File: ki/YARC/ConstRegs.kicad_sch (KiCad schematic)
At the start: 11 parts, among them U91 74HC245, U92 74LS157, U93 74LS32, U94 74HC245, U95 74HC245, U96 74LS32, U96A1 74LS32, U96B1 74LS32, U97 74HC00, U98 74HC245, U99 74HC245

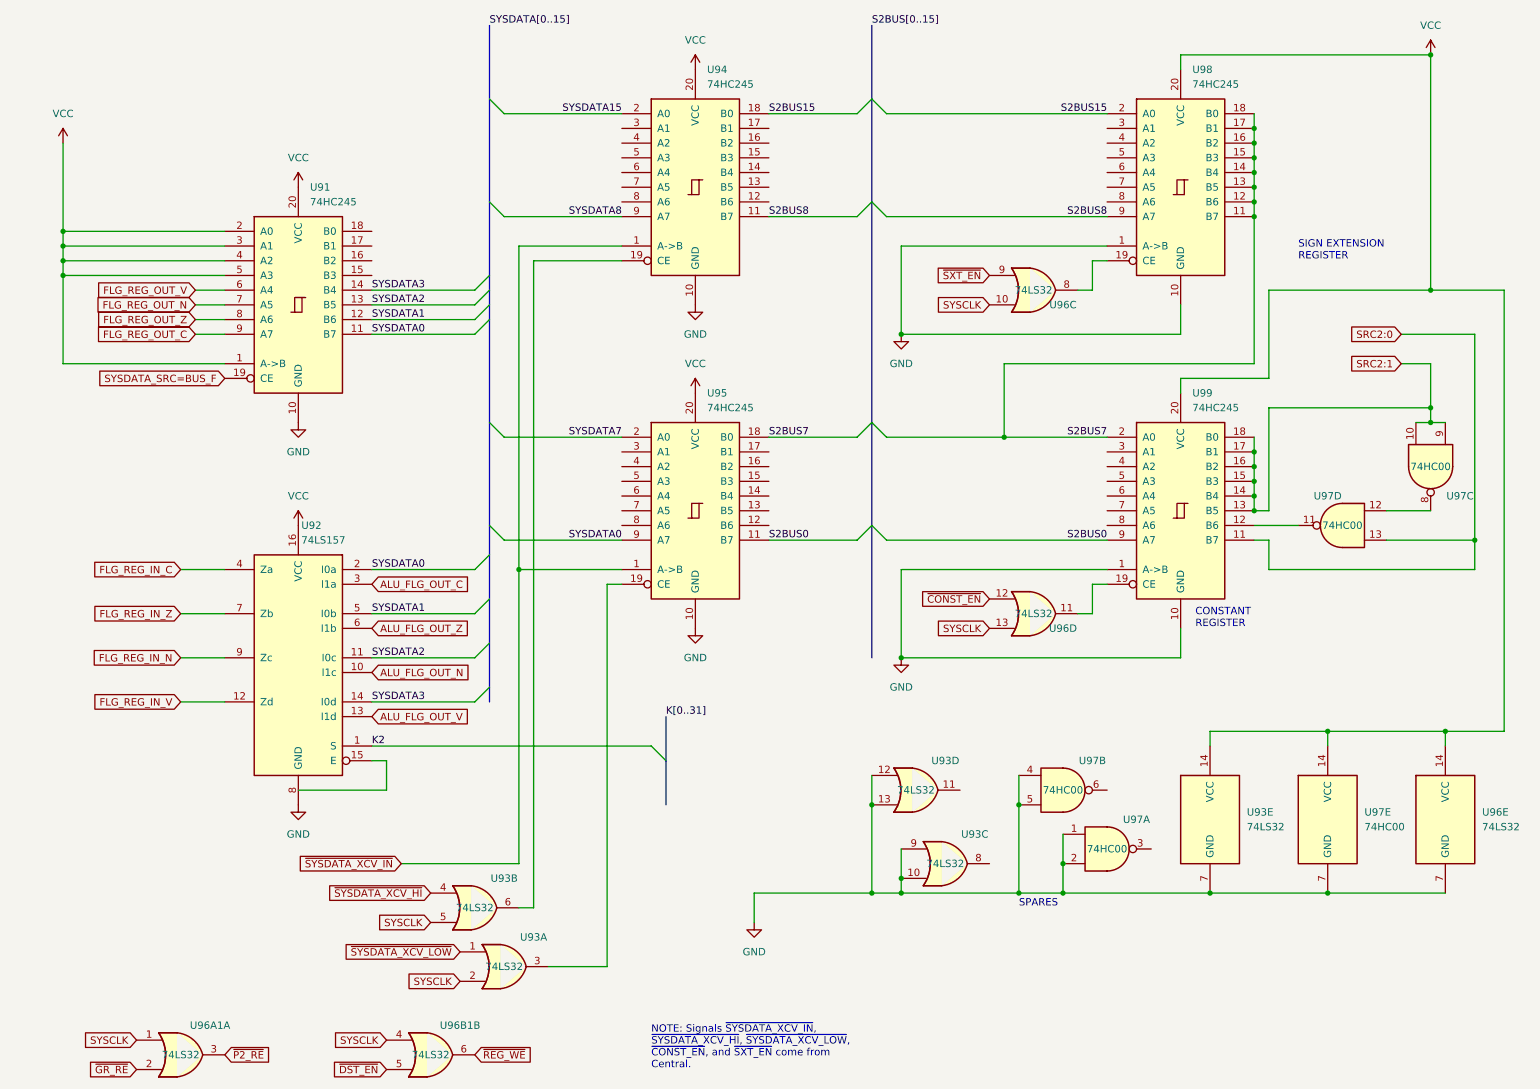
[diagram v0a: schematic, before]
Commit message: Various corrections and minor improvements
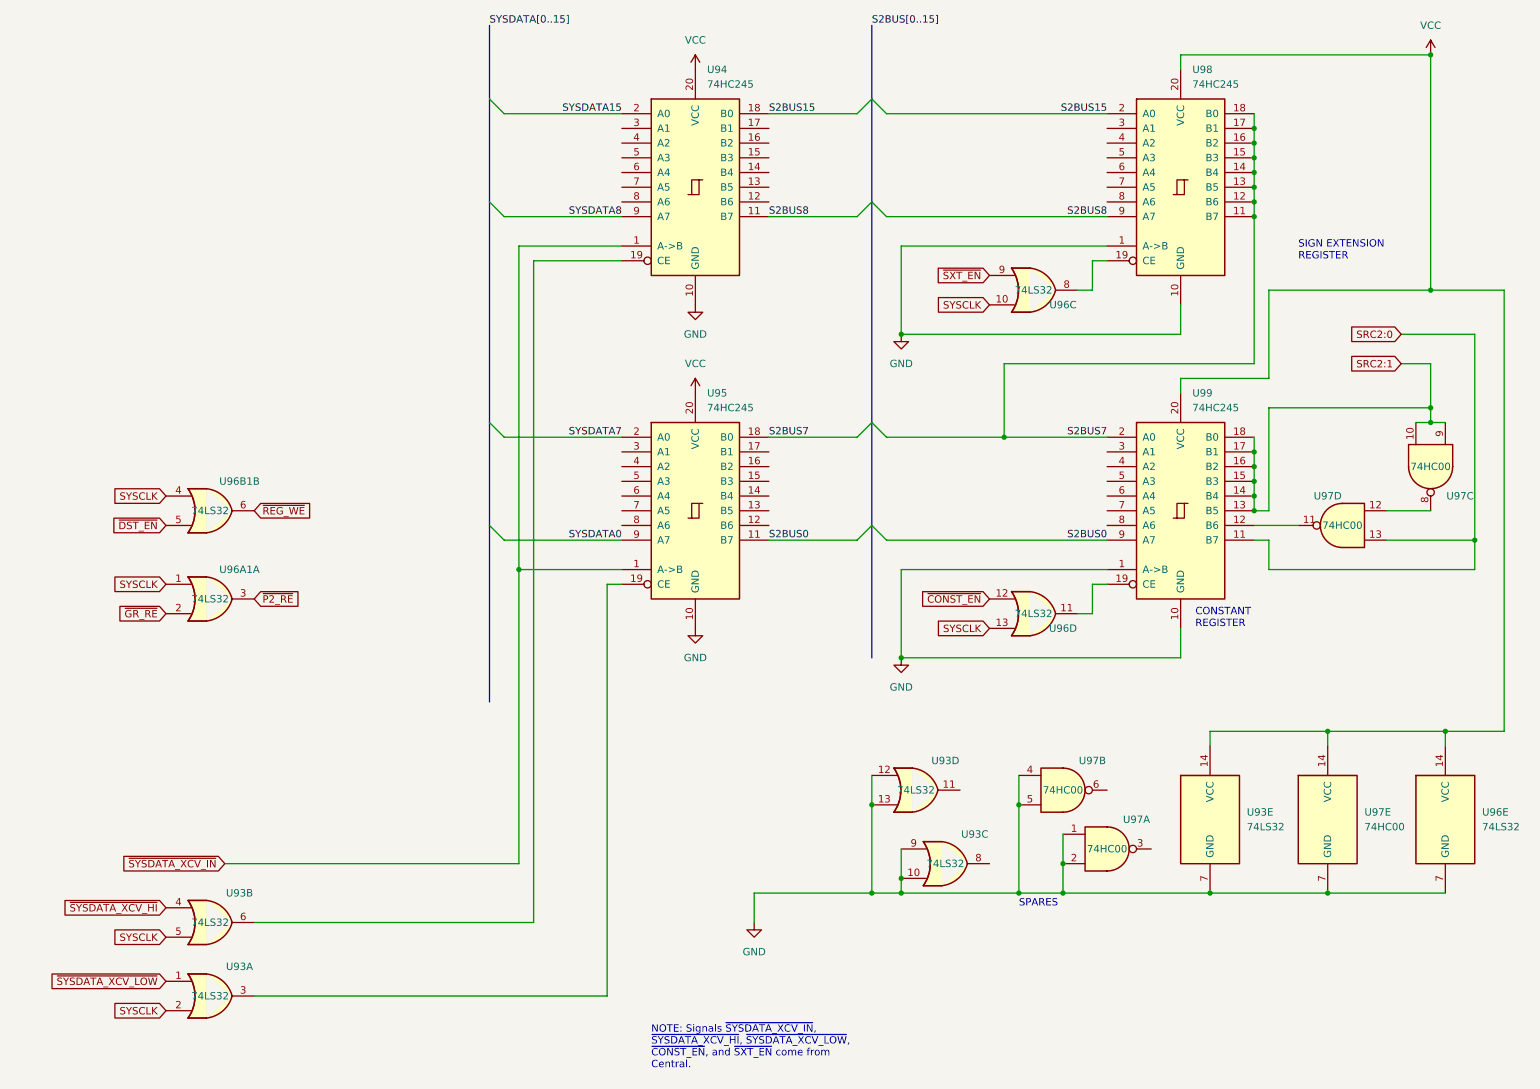
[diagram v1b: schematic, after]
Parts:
- removed U91: 74HC245, symbol 74xx:74HC245
- removed U92: 74LS157, symbol 74xx:74LS157
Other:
- moved on the sheet: U93A, U93B, U96A1A, U96B1B
